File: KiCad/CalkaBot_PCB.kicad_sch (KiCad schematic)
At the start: 12 parts, among them J1 Conn_01x03_Pin, J2 Conn_01x03_Pin, J3 Conn_01x03_Pin, M1 Motor_Right, M2 Motor_Left, Q1 KTIR0711S, Q2 KTIR0711S, SW1 SW_DIP_x04, U1 TB6612FNG, U2 L7805

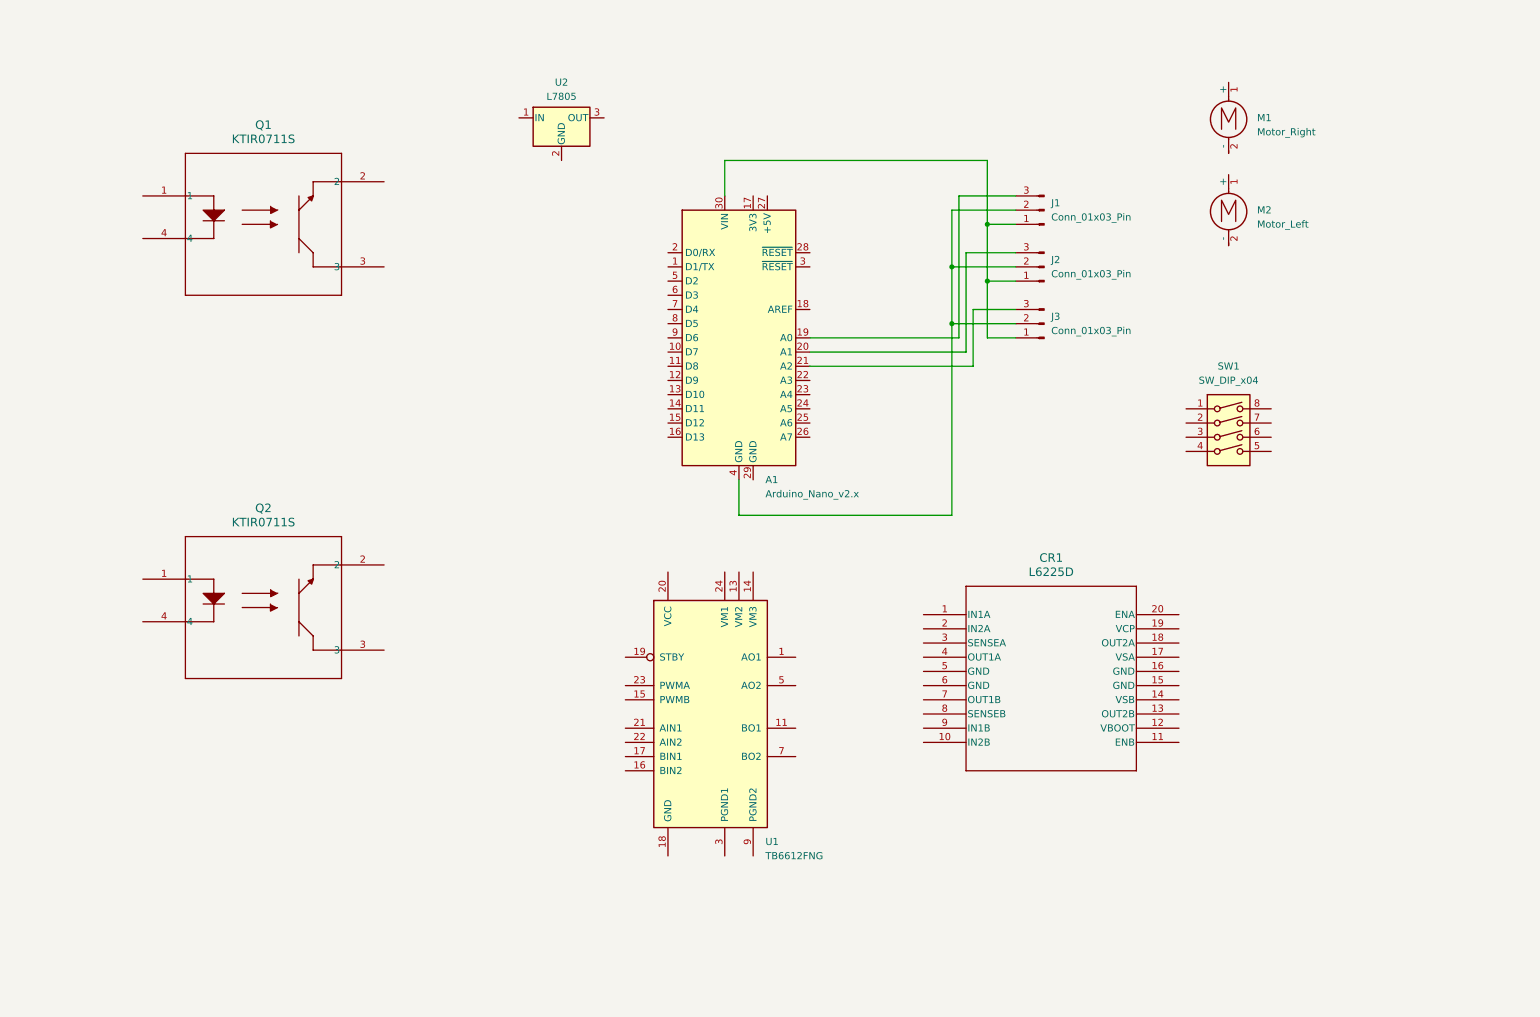
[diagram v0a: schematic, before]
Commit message: working on PCB + changes within NX for project review
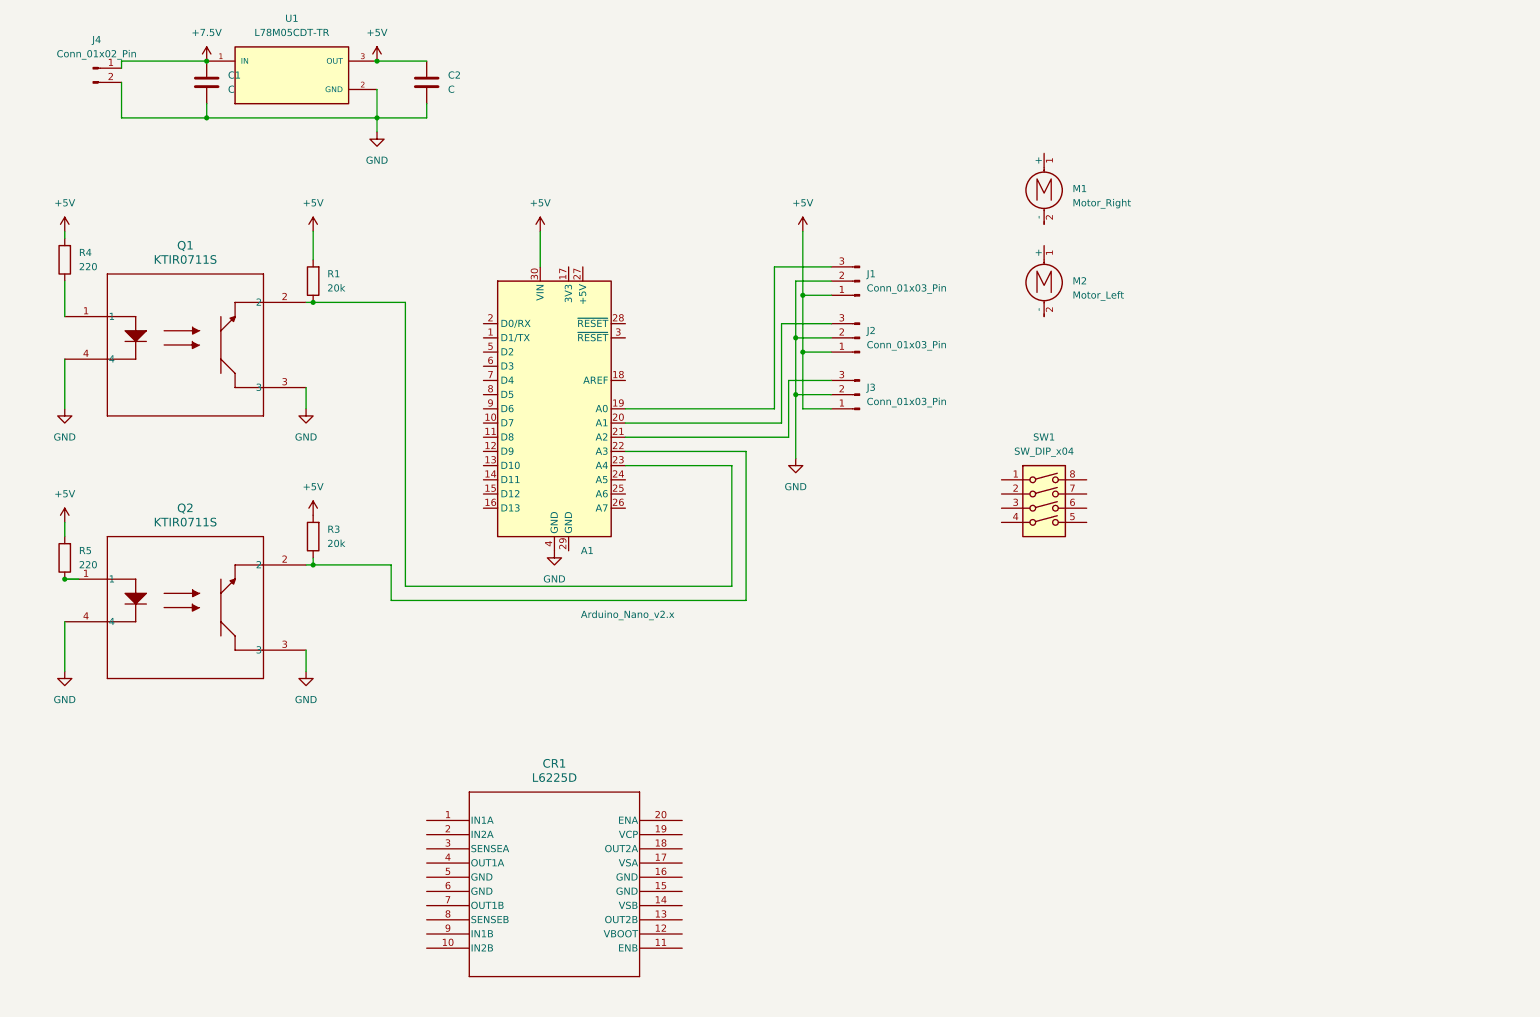
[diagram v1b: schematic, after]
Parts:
- removed U1: TB6612FNG, Package_SO:SSOP-24_5.3x8.2mm_P0.65mm, symbol Driver_Motor:TB6612FNG
- removed U2: L7805, Package_TO_SOT_THT:TO-220-3_Horizontal_TabDown, symbol Regulator_Linear:L7805
- added C1, C2: C, symbol Device:C
- added J4: Conn_01x02_Pin, Connector_PinSocket_1.00mm:PinSocket_1x02_P1.00mm_Vertical, symbol Connector:Conn_01x02_Pin
- added R1, R3: 20k, Resistor_SMD:R_0805_2012Metric_Pad1.20x1.40mm_HandSolder, symbol Device:R
- added R4, R5: 220, Resistor_SMD:R_0805_2012Metric_Pad1.20x1.40mm_HandSolder, symbol Device:R
- added U1: L78M05CDT-TR, L78M05CDT-TR:VREG_L78M05CDT-TR, symbol L78M05CDT-TR:L78M05CDT-TR
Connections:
- net at Q1.1: now also R4.1
- net at Q1.2: now also A1.23 (A4), R1.1
- net GND: now reaches Q1.3
- net GND: now also A1.4 (GND), J1.2 (Pin_2), J2.2 (Pin_2), J3.2 (Pin_2), Q1.4, Q2.3, Q2.4, C1.2, C2.2, J4.2 (Pin_2), U1.2 (GND)
- net +5V: now reaches A1.30 (VIN), J1.1 (Pin_1), J2.1 (Pin_1), J3.1 (Pin_1)
- net +5V: now also C2.1, R1.2, R3.2, R4.2, R5.2, U1.3 (OUT)
- net at Q2.1: now also R5.1
- net at Q2.2: now also A1.22 (A3), R3.1
- new net +7.5V: C1.1, J4.1 (Pin_1), U1.1 (IN)
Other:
- moved on the sheet: A1, CR1, J1, J2, J3, M1, M2, Q1, Q2, SW1

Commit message: w trakcie ukladania elementow
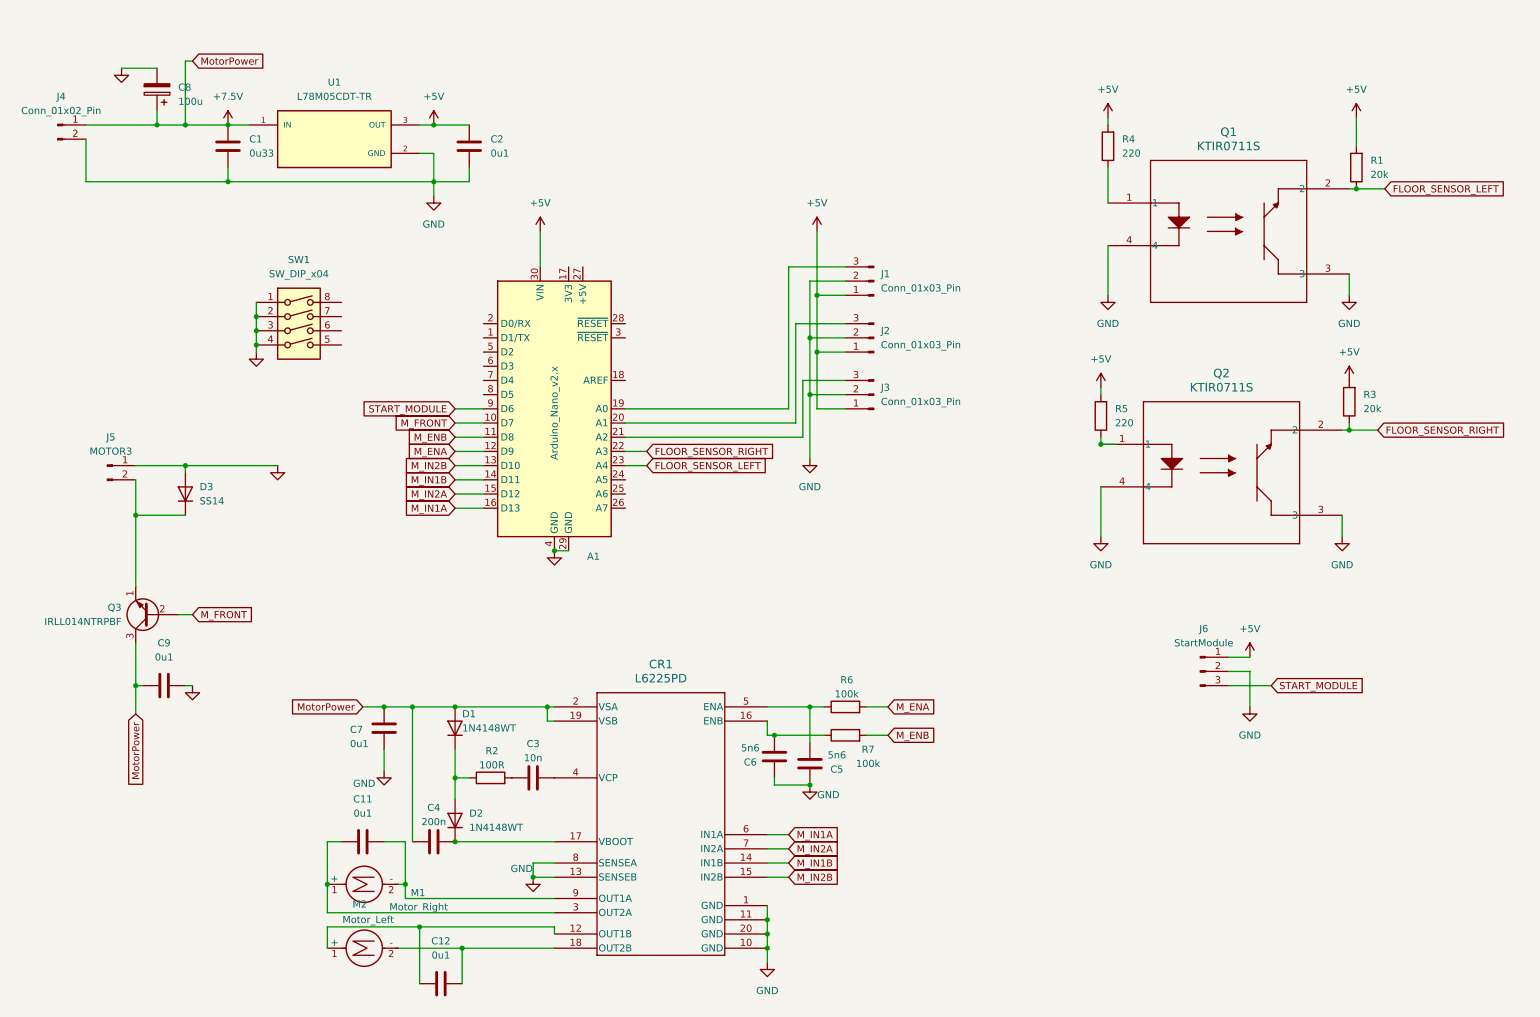
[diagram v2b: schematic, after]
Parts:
- added C11, C12, C7, C9: 0u1, Capacitor_SMD:C_0805_2012Metric_Pad1.18x1.45mm_HandSolder, symbol Device:C
- added C3: 10n, Capacitor_SMD:C_0805_2012Metric_Pad1.18x1.45mm_HandSolder, symbol Device:C
- added C4: 200n, Capacitor_SMD:C_0805_2012Metric_Pad1.18x1.45mm_HandSolder, symbol Device:C
- added C5, C6: 5n6, Capacitor_SMD:C_0805_2012Metric_Pad1.18x1.45mm_HandSolder, symbol Device:C
- added C8: 100u, Capacitor_SMD:CP_Elec_8x10.5, symbol Device:C_Polarized
- added D1, D2: 1N4148WT, Diode_SMD:D_SOD-523, symbol Diode:1N4148WT
- added D3: SS14, Diode_SMD:D_SMA_Handsoldering, symbol Device:D
- added J5: MOTOR3, Connector_PinHeader_2.54mm:PinHeader_1x02_P2.54mm_Vertical, symbol Connector:Conn_01x02_Pin
- added J6: StartModule, Connector_PinHeader_2.54mm:PinHeader_1x03_P2.54mm_Vertical, symbol Connector:Conn_01x03_Pin
- added Q3: IRLL014NTRPBF, Package_TO_SOT_SMD:SOT-223, symbol Transistor_BJT:BC107
- added R2: 100R, Resistor_SMD:R_0805_2012Metric_Pad1.20x1.40mm_HandSolder, symbol Device:R
- added R6, R7: 100k, Resistor_SMD:R_0805_2012Metric_Pad1.20x1.40mm_HandSolder, symbol Device:R
- C1: value C -> 0u33; footprint (none) -> Capacitor_SMD:C_0805_2012Metric_Pad1.18x1.45mm_HandSolder
- C2: value C -> 0u1; footprint (none) -> Capacitor_SMD:C_0805_2012Metric_Pad1.18x1.45mm_HandSolder
- CR1: value L6225D -> L6225PD; footprint SO-20_STM -> Package_SO:SO-20-1EP_7.52x12.825mm_P1.27mm_EP6.045x12.09mm_Mask3.56x4.47mm_ThermalVias
- J4: footprint Connector_PinSocket_1.00mm:PinSocket_1x02_P1.00mm_Vertical -> Connector_PinHeader_2.54mm:PinHeader_1x02_P2.54mm_Vertical
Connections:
- net +5V: now also J6.1 (Pin_1)
- net +7.5V: now also CR1.19 (VSB), CR1.2 (VSA), C4.1, C7.1, C8.1, C9.1, D1.2 (A), Q3.3 (C)
- net GND: now also A1.29 (GND), CR1.1 (GND), CR1.10 (GND), CR1.11 (GND), CR1.13 (SENSEB), CR1.20 (GND), CR1.8 (SENSEA), SW1.1, SW1.2, SW1.3, SW1.4, C5.1, C6.1, C7.2, C8.2, C9.2, D3.2 (A), J5.1 (Pin_1), J6.2 (Pin_2)
- net FLOOR_SENSOR_LEFT: now reaches A1.23 (A4), Q1.2, R1.1
- net at CR1.12 (OUT1B): now also M2.1 (+), C12.2
- net M_IN1B: now reaches CR1.14 (IN1B)
- net M_IN1B: now also A1.14 (D11)
- net M_IN2B: now reaches CR1.15 (IN2B)
- net M_IN2B: now also A1.13 (D10)
- net at CR1.16 (ENB): now also C6.2, R7.1
- net at CR1.17 (VBOOT): now also C4.2, D2.1 (K)
- net at CR1.18 (OUT2B): now also M2.2 (-), C12.1
- net at CR1.3 (OUT2A): now also M1.1 (+), C11.2
- net at CR1.4 (VCP): now also C3.2
- net at CR1.5 (ENA): now also C5.2, R6.1
- net M_IN1A: now reaches CR1.6 (IN1A)
- net M_IN1A: now also A1.16 (D13)
- net M_IN2A: now reaches CR1.7 (IN2A)
- net M_IN2A: now also A1.15 (D12)
- net at CR1.9 (OUT1A): now also M1.2 (-), C11.1
- net FLOOR_SENSOR_RIGHT: now reaches A1.22 (A3), Q2.2, R3.1
- net M_FRONT: now reaches A1.10 (D7)
- net M_FRONT: now also Q3.2 (B)
- net M_ENB: now reaches A1.11 (D8)
- net M_ENB: now also R7.2
- net M_ENA: now reaches A1.12 (D9)
- net M_ENA: now also R6.2
- net START_MODULE: now reaches A1.9 (D6)
- net START_MODULE: now also J6.3 (Pin_3)
- new net: D1.1 (K), D2.2 (A), R2.1
- new net: D3.1 (K), J5.2 (Pin_2), Q3.1 (E)
- new net: C3.1, R2.2
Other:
- moved on the sheet: C1, C2, CR1, J1, J2, J3, J4, M1, M2, Q1, Q2, R1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

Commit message: PCB finished ready to send
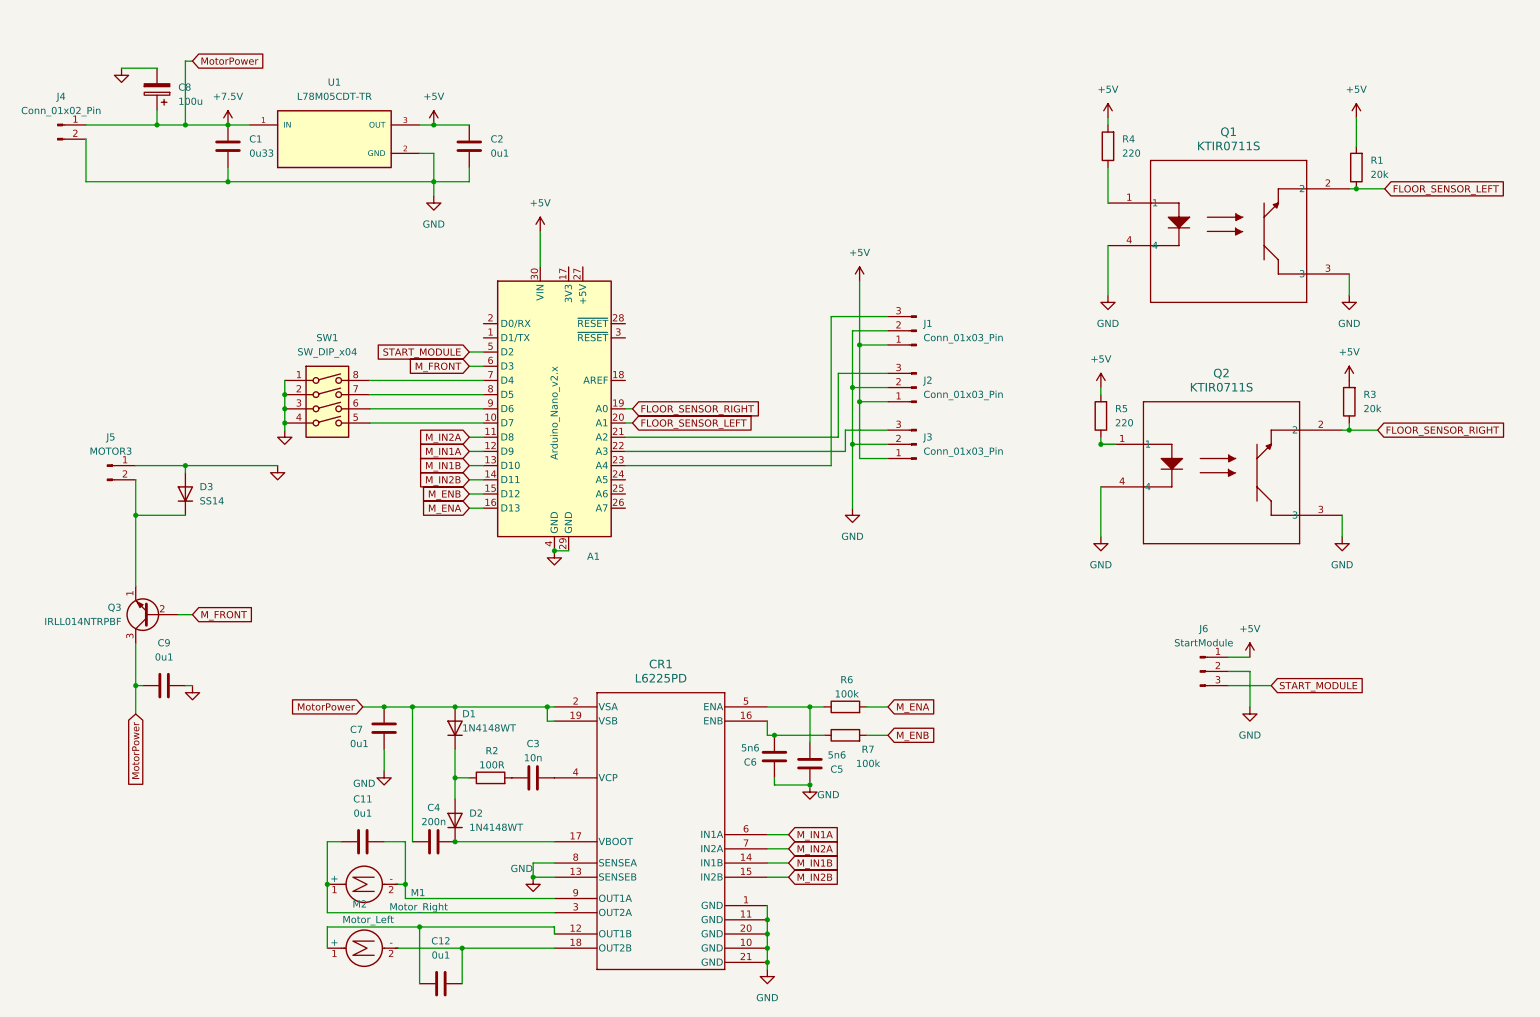
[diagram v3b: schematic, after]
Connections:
- net FLOOR_SENSOR_LEFT: now also A1.20 (A1); no longer A1.23 (A4)
- net FLOOR_SENSOR_RIGHT: now also A1.19 (A0); no longer A1.22 (A3)
- net GND: now also CR1.21 (GND)
- net M_ENA: now also A1.16 (D13); no longer A1.12 (D9)
- net M_ENB: now also A1.15 (D12); no longer A1.11 (D8)
- net M_FRONT: now also A1.6 (D3); no longer A1.10 (D7)
- net M_IN1A: now also A1.12 (D9); no longer A1.16 (D13)
- net M_IN1B: now also A1.13 (D10); no longer A1.14 (D11)
- net M_IN2A: now also A1.11 (D8); no longer A1.15 (D12)
- net M_IN2B: now also A1.14 (D11); no longer A1.13 (D10)
- net START_MODULE: now also A1.5 (D2); no longer A1.9 (D6)
- net at J1.3 (Pin_3): now also A1.23 (A4); no longer A1.19 (A0)
- net at SW1.5: now also A1.10 (D7)
- net at SW1.6: now also A1.9 (D6)
- net at SW1.7: now also A1.8 (D5)
- net at SW1.8: now also A1.7 (D4)
- net at J2.3 (Pin_3): now also A1.21 (A2); no longer A1.20 (A1)
- net at J3.3 (Pin_3): now also A1.22 (A3); no longer A1.21 (A2)
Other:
- moved on the sheet: J1, J2, J3, SW1
